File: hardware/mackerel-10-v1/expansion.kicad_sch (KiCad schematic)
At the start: 2 parts, among them J9 Conn_02x20_Odd_Even

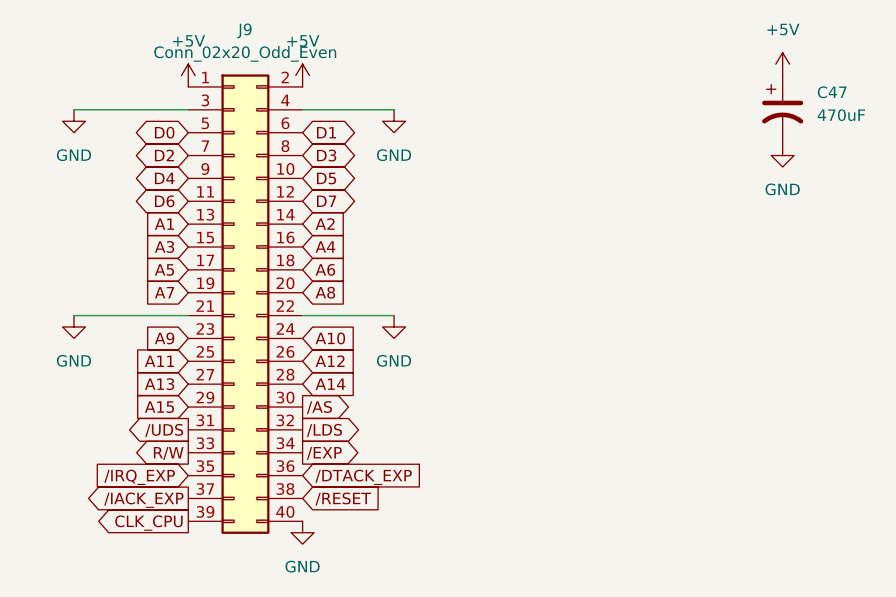
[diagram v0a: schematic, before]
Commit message: Mack-10 v1 fully routed
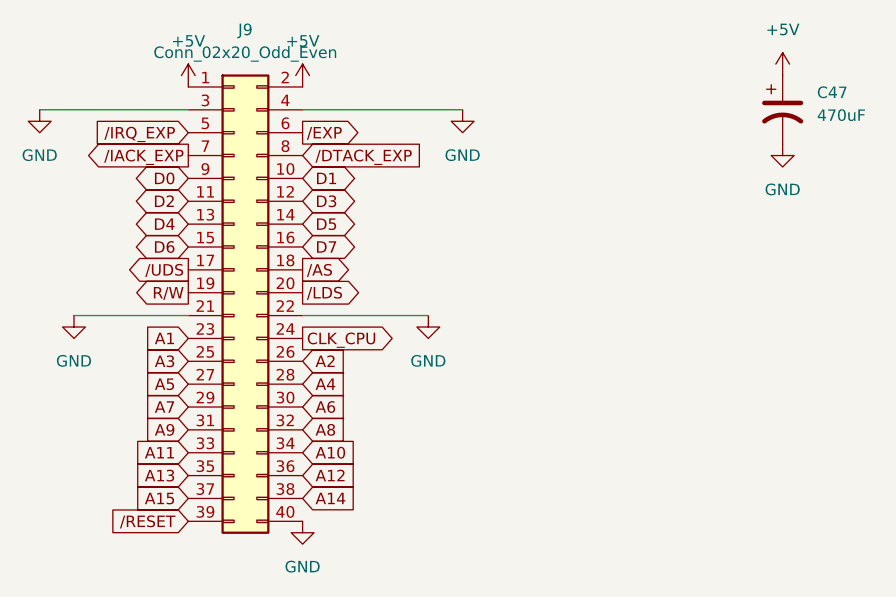
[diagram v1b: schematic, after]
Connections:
- net A1: now also J9.23 (Pin_23); no longer J9.13 (Pin_13)
- net A10: now also J9.34 (Pin_34); no longer J9.24 (Pin_24)
- net A11: now also J9.33 (Pin_33); no longer J9.25 (Pin_25)
- net A12: now also J9.36 (Pin_36); no longer J9.26 (Pin_26)
- net A13: now also J9.35 (Pin_35); no longer J9.27 (Pin_27)
- net A14: now also J9.38 (Pin_38); no longer J9.28 (Pin_28)
- net A15: now also J9.37 (Pin_37); no longer J9.29 (Pin_29)
- net A2: now also J9.26 (Pin_26); no longer J9.14 (Pin_14)
- net A3: now also J9.25 (Pin_25); no longer J9.15 (Pin_15)
- net A4: now also J9.28 (Pin_28); no longer J9.16 (Pin_16)
- net A5: now also J9.27 (Pin_27); no longer J9.17 (Pin_17)
- net A6: now also J9.30 (Pin_30); no longer J9.18 (Pin_18)
- net A7: now also J9.29 (Pin_29); no longer J9.19 (Pin_19)
- net A8: now also J9.32 (Pin_32); no longer J9.20 (Pin_20)
- net A9: now also J9.31 (Pin_31); no longer J9.23 (Pin_23)
- net CLK_CPU: now also J9.24 (Pin_24); no longer J9.39 (Pin_39)
- net D0: now also J9.9 (Pin_9); no longer J9.5 (Pin_5)
- net D1: now also J9.10 (Pin_10); no longer J9.6 (Pin_6)
- net D2: now also J9.11 (Pin_11); no longer J9.7 (Pin_7)
- net D3: now also J9.12 (Pin_12); no longer J9.8 (Pin_8)
- net D4: now also J9.13 (Pin_13); no longer J9.9 (Pin_9)
- net D5: now also J9.14 (Pin_14); no longer J9.10 (Pin_10)
- net D6: now also J9.15 (Pin_15); no longer J9.11 (Pin_11)
- net D7: now also J9.16 (Pin_16); no longer J9.12 (Pin_12)
- net R/W: now also J9.19 (Pin_19); no longer J9.33 (Pin_33)
- net /AS: now also J9.18 (Pin_18); no longer J9.30 (Pin_30)
- net /DTACK_EXP: now also J9.8 (Pin_8); no longer J9.36 (Pin_36)
- net /EXP: now also J9.6 (Pin_6); no longer J9.34 (Pin_34)
- net /IACK_EXP: now also J9.7 (Pin_7); no longer J9.37 (Pin_37)
- net /IRQ_EXP: now also J9.5 (Pin_5); no longer J9.35 (Pin_35)
- net /LDS: now also J9.20 (Pin_20); no longer J9.32 (Pin_32)
- net /RESET: now also J9.39 (Pin_39); no longer J9.38 (Pin_38)
- net /UDS: now also J9.17 (Pin_17); no longer J9.31 (Pin_31)
